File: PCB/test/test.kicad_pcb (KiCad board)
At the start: 2 copper layers, 41.6 x 86.8 mm, 178 parts, among them U1 STM32WBxx_QFN48, U2 USBLC6-2SC6, U3 LD3985M33R, X1 NX2016_32MHz, X2 NX2012_32K768Hz

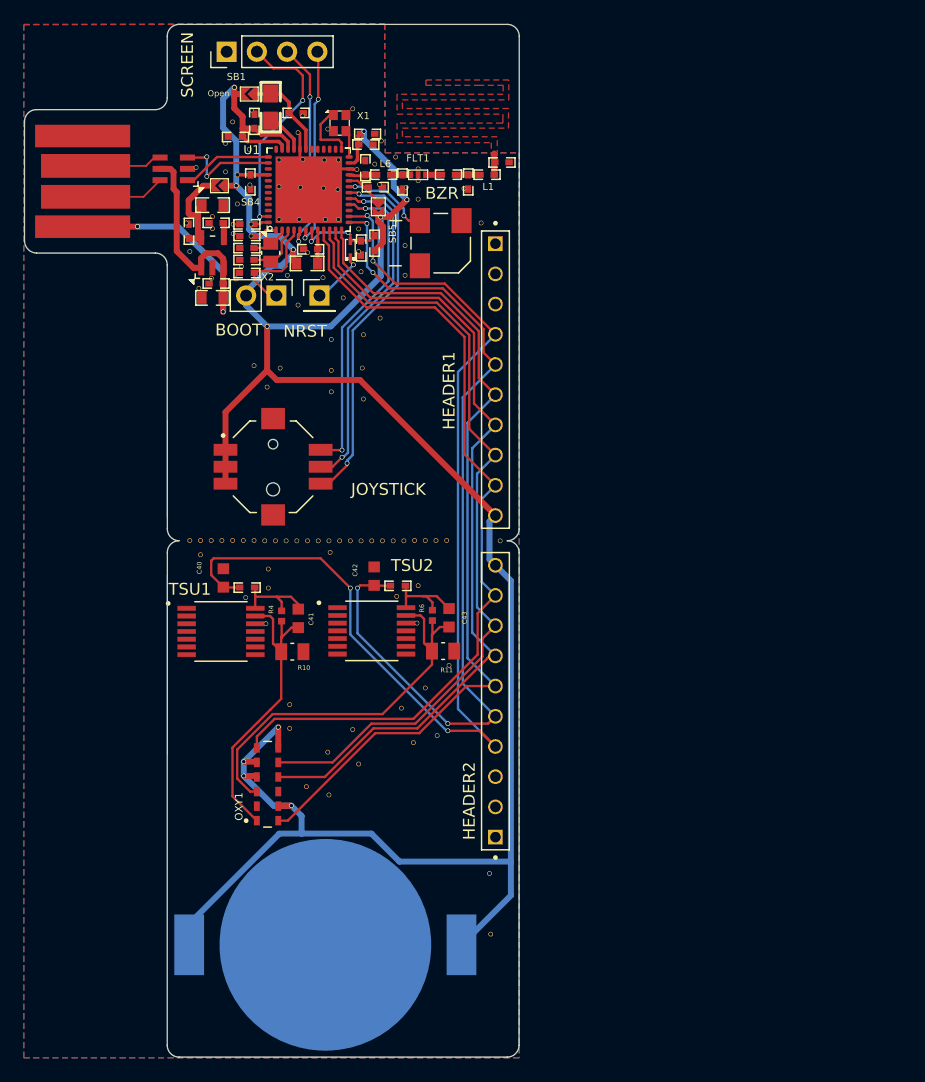
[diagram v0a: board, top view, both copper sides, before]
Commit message: réduction taille
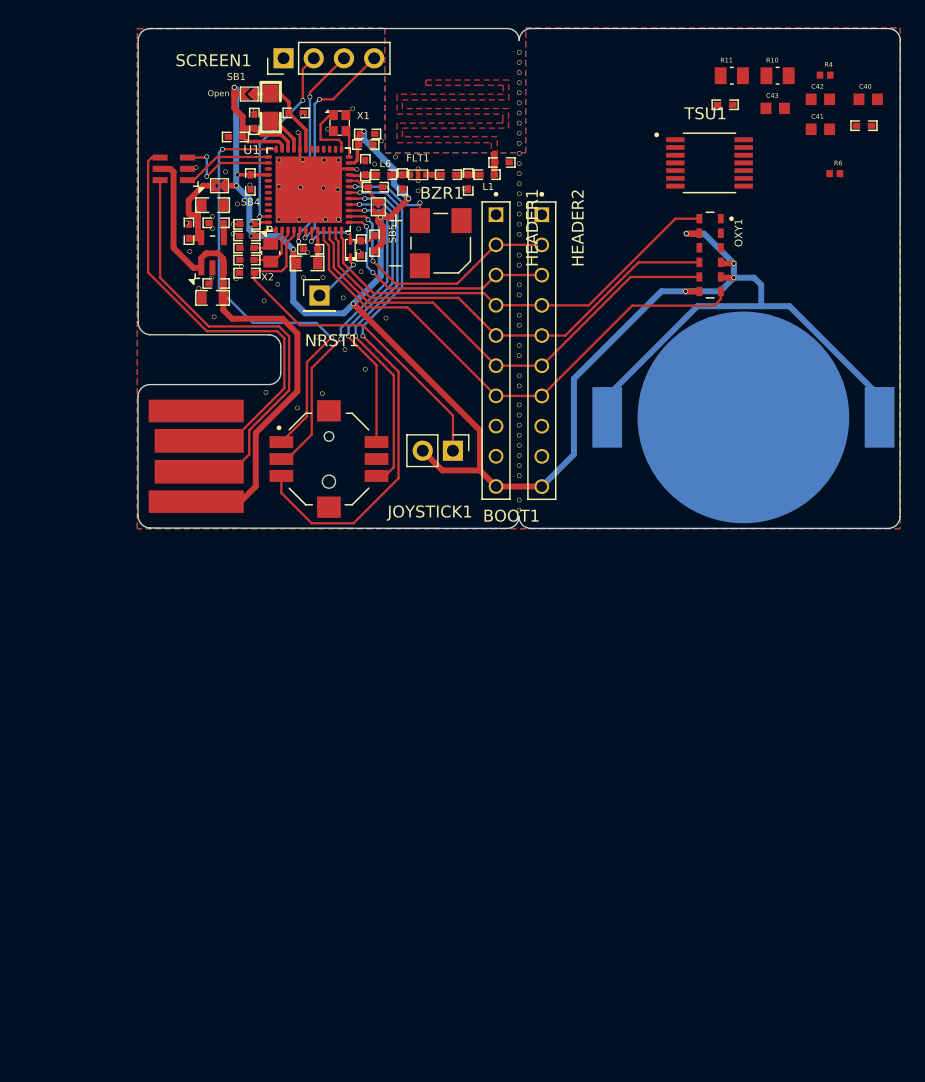
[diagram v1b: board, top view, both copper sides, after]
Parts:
- removed the ? at (135.8, 122.6)
- removed the ? at (133.4, 138.4)
- removed the ? at (139.6, 110.7)
- removed the ? at (134.0, 122.6)
- removed the ? at (145.7, 122.6)
- removed the ? at (136.9, 110.1)
- removed the ? at (131.3, 122.6)
- removed the ? at (136.9, 105.7)
- removed the ? at (132.6, 108.1)
- removed the ? at (132.2, 122.6)
- removed the ? at (145.8, 139.0)
- removed the ? at (141.2, 122.6)
- removed the ? at (127.7, 122.6)
- removed the ? at (128.6, 87.4)
- removed the ? at (151.1, 122.6)
- removed the ? at (144.2, 126.4)
- removed the ? at (134.8, 143.3)
- removed the ? at (136.7, 122.6)
- removed the ? at (139.5, 108.1)
- removed the ? at (141.0, 103.9)
- removed the ? at (133.2, 100.3)
- removed the ? at (143.2, 92.9)
- removed the ? at (142.8, 136.7)
- removed the ? at (144.1, 129.6)
- removed the ? at (140.3, 122.6)
- removed the ? at (139.6, 105.3)
- removed the ? at (130.4, 107.9)
- removed the ? at (143.9, 122.6)
- removed the ? at (136.6, 140.4)
- removed the ? at (125.0, 122.6)
- removed the ? at (140.9, 92.7)
- removed the ? at (144.2, 93.9)
- removed the ? at (142.4, 127.3)
- removed the ? at (146.6, 122.6)
- removed the ? at (131.5, 109.7)
- removed the ? at (143.1, 97.8)
- removed the ? at (129.7, 127.4)
- removed the ? at (142.1, 122.6)
- removed the ? at (130.0, 89.7)
- removed the ? at (128.0, 89.2)
- removed the ? at (143.0, 122.6)
- removed the ? at (149.5, 95.9)
- removed the ? at (143.8, 139.6)
- removed the ? at (144.8, 135.0)
- removed the ? at (136.9, 108.3)
- removed the ? at (136.8, 123.6)
- removed the ? at (131.6, 125.0)
- removed the ? at (130.4, 122.6)
- removed the ? at (131.6, 126.6)
- removed the ? at (129.5, 122.6)
- removed the ? at (133.4, 136.4)
- removed the ? at (136.7, 144.0)
- removed the ? at (137.6, 122.6)
- removed the ? at (144.8, 122.6)
- removed the ? at (131.4, 129.6)
- removed the ? at (143.1, 100.3)
- removed the ? at (150.2, 150.6)
- removed the ? at (126.8, 122.6)
- removed the ? at (138.5, 122.6)
- removed the ? at (150.3, 155.7)
- removed the ? at (138.7, 138.5)
- removed the ? at (139.2, 141.4)
- removed the ? at (139.4, 122.6)
- removed the ? at (146.8, 133.1)
- removed the ? at (134.1, 102.8)
- removed the ? at (134.9, 122.6)
- removed the ? at (133.1, 122.6)
- removed the ? at (128.6, 122.6)
- removed the ? at (125.9, 123.8)
- removed the ? at (125.9, 122.6)
- removed JOYSTICK: JS1400AFQ, JS1400AFQ:SW_JS1400AFQ
- removed TSU2: TSU104IPT, TSU104IPT:SOP65P640X120-14N
- added ?: , , F.Cu at (134.1, 111.5)
- added ?: , , F.Cu at (152.7, 83.2)
- added ?: , , F.Cu at (152.7, 111.2)
- added ?: , , F.Cu at (144.2, 93.2)
- added ?: , , F.Cu at (152.7, 82.4)
- added ?: , , F.Cu at (152.7, 92.6)
- added ?: , , F.Cu at (152.7, 95.2)
- added ?: , , F.Cu at (138.1, 106.5)
- added ?: , , F.Cu at (136.2, 110.2)
- added ?: , , F.Cu at (152.7, 112.9)
- added ?: , , F.Cu at (152.7, 85.8)
- added ?: , , F.Cu at (139.8, 108.2)
- added ?: , , F.Cu at (132.4, 101.0)
- added ?: , , F.Cu at (152.7, 89.2)
- added ?: , , F.Cu at (152.7, 109.6)
- added ?: , , F.Cu at (134.6, 100.5)
- added ?: , , F.Cu at (152.7, 86.7)
- added ?: , , F.Cu at (152.7, 103.7)
- added ?: , , F.Cu at (152.7, 104.5)
- added ?: , , F.Cu at (152.7, 90.9)
- added ?: , , F.Cu at (152.7, 114.6)
- added ?: , , F.Cu at (152.7, 112.0)
- added ?: , , F.Cu at (152.7, 93.5)
- added ?: , , F.Cu at (152.7, 108.8)
- added ?: , , F.Cu at (152.7, 90.0)
- added ?: , , F.Cu at (152.7, 85.0)
- added ?: , , F.Cu at (131.2, 102.5)
- added ?: , , F.Cu at (152.7, 96.0)
- added ?: , , F.Cu at (152.7, 115.5)
- added ?: , , F.Cu at (141.5, 103.9)
- added ?: , , F.Cu at (131.4, 110.2)
- added ?: , , F.Cu at (152.7, 94.3)
- added ?: , , F.Cu at (152.7, 84.1)
- added ?: , , F.Cu at (152.7, 88.3)
- added ?: , , F.Cu at (152.7, 99.5)
- added ?: , , F.Cu at (152.7, 98.6)
- added ?: , , F.Cu at (152.7, 107.0)
- added ?: , , F.Cu at (135.7, 105.5)
- added ?: , , F.Cu at (127.0, 103.8)
- added ?: , , F.Cu at (152.7, 120.0)
- added ?: , , F.Cu at (152.7, 91.8)
- added ?: , , F.Cu at (152.7, 101.1)
- added ?: , , F.Cu at (152.7, 81.5)
- added ?: , , F.Cu at (152.7, 119.2)
- added ?: , , F.Cu at (152.7, 113.8)
- added ?: , , F.Cu at (152.7, 96.8)
- added ?: , , F.Cu at (152.7, 87.5)
- added ?: , , F.Cu at (152.7, 102.0)
- added ?: , , F.Cu at (152.7, 116.3)
- added ?: , , F.Cu at (152.7, 106.2)
- added ?: , , F.Cu at (152.7, 117.2)
- added JOYSTICK1: JS1400AFQ, JS1400AFQ:SW_JS1400AFQ, F.Cu at (136.7, 115.8)
- moved C40 67.5 mm to (182.0, 85.5), turned to 0 degrees
- moved R3 64.8 mm to (181.7, 87.7), turned to 0 degrees
- moved R4 64.5 mm to (178.4, 83.5), turned to 0 degrees
- moved R10 63.3 mm to (174.4, 83.5)
- moved C41 60.2 mm to (178.0, 88.0), turned to 0 degrees
- moved OXY1 58.0 mm to (168.8, 98.6), turned to -90 degrees
- moved TSU1 56.9 mm to (168.7, 90.8)
- moved BATTERY1 56.6 mm to (171.6, 112.2)
- moved C42 54.9 mm to (178.0, 85.5), turned to 0 degrees
- moved R11 54.1 mm to (170.6, 83.5)
- moved HEADER2 52.5 mm to (154.6, 95.2), turned to -90 degrees
- moved C43 50.9 mm to (174.2, 86.3), turned to 0 degrees
- moved R6 50.2 mm to (179.2, 91.8), turned to 0 degrees
- moved R5 48.9 mm to (170.0, 86.0), turned to 0 degrees
- moved USB1 25.0 mm to (120.6, 115.5)
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- renumbered BOOT to BOOT1, BZR to BZR1, NRST to NRST1, SCREEN to SCREEN1
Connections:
- HEADER1 pad 2: unconnected-(HEADER1-Pad2) -> PA5
- HEADER1 pad 3: unconnected-(HEADER1-Pad3) -> PA4
- HEADER1 pad 4: PA5 -> PA3
- HEADER1 pad 5: PA4 -> PA2
- HEADER1 pad 6: PA3 -> PA1
- HEADER1 pad 7: PA2 -> PA0
- HEADER1 pad 8: PA1 -> unconnected-(HEADER1-Pad8)
- HEADER1 pad 9: PA0 -> unconnected-(HEADER1-Pad9)
- HEADER2 pad 2: unconnected-(HEADER2-Pad2) -> PA5
- HEADER2 pad 3: unconnected-(HEADER2-Pad3) -> PA4
- HEADER2 pad 4: PA5 -> PA3
- HEADER2 pad 5: PA4 -> PA2
- HEADER2 pad 6: PA3 -> PA1
- HEADER2 pad 7: PA2 -> PA0
- HEADER2 pad 8: PA1 -> unconnected-(HEADER2-Pad8)
- HEADER2 pad 9: PA0 -> unconnected-(HEADER2-Pad9)
- TSU1 pad 10: (no net) -> GND
- TSU1 pad 8: (no net) -> Net-(C43-Pad2)
- TSU1 pad 9: (no net) -> Net-(C43-Pad1)
- U1 pad 15: unconnected-(U1-Pad15) -> PA6
- U1 pad 36: unconnected-(U1-Pad36) -> PA10
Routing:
- net PA5: track 92.5 -> 21.7 mm, vias 4 -> 2
- net PA4: track 74.0 -> 20.9 mm, vias 4 -> 2
- net PA10: track 0.00 -> 38.0 mm, vias 0 -> 2
- net PA3: track 71.9 -> 37.3 mm
- net Net-(C43-Pad1): track 33.9 -> 0.00 mm
- net 3V3: track 210.3 -> 178.8 mm
- net Net-(U2-Pad4): track 6.55 -> 37.4 mm
- net PA2: track 68.8 -> 38.4 mm
- net Net-(U2-Pad6): track 6.84 -> 37.2 mm
- net PA6: track 0.00 -> 27.9 mm, vias 0 -> 2
- net PA1: track 67.6 -> 40.6 mm
- net Net-(C41-Pad1): track 25.8 -> 0.00 mm
- net PA0: track 69.0 -> 44.9 mm
- net Net-(BOOT1-Pad1): track 9.23 -> 31.2 mm
- net PA9: track 30.8 -> 44.2 mm
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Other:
- board size 41.6 x 86.8 mm -> 64.1 x 42 mm
